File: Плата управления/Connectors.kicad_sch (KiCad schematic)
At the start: 9 parts, among them J1 A, J2 B, J3 C, J4 CAN2, J5 Conn_02x07_Odd_Even, J6 CAN1, J7 RS-485, J8 Conn_02x10_Odd_Even, J9 Inputs

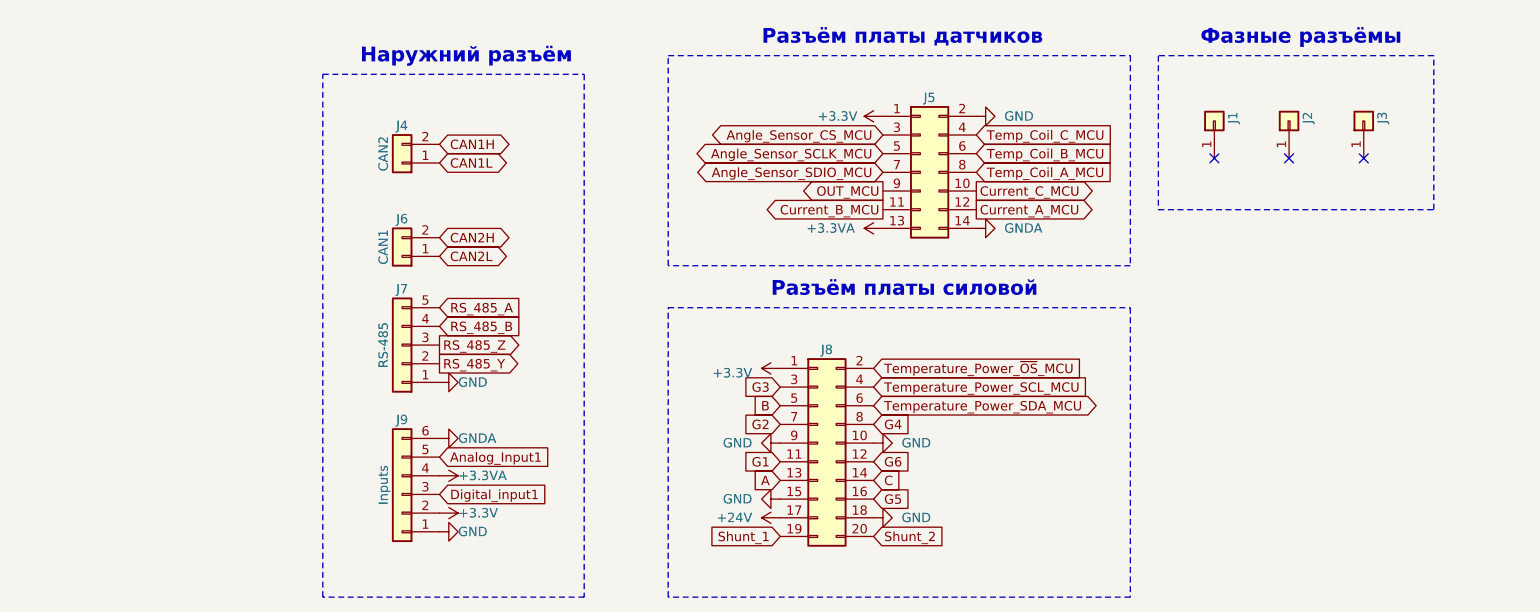
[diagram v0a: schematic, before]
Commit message: Версия под отчёт
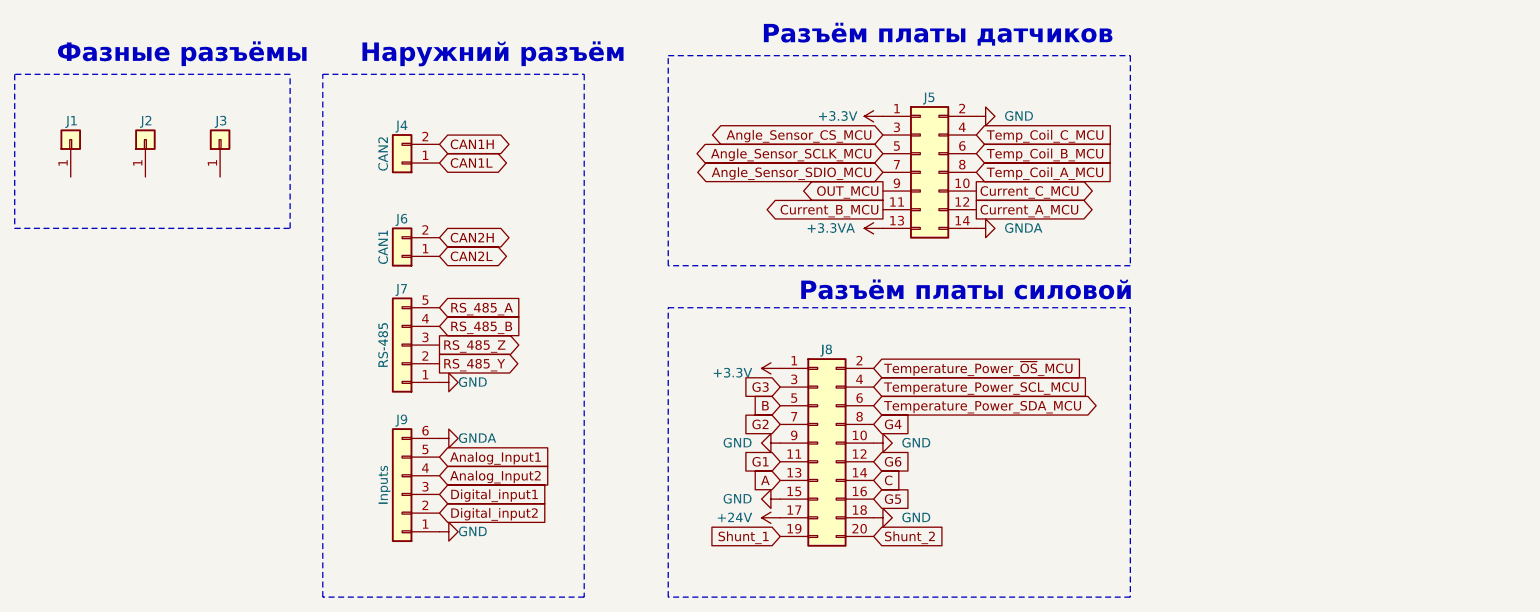
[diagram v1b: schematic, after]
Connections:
- net +3.3V: no longer J9.2 (Pin_2)
- net +3.3VA: no longer J9.4 (Pin_4)
- new net Analog_Input2: J9.4 (Pin_4)
- new net Digital_input2: J9.2 (Pin_2)
- no-connect marks 3 -> 0
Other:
- moved on the sheet: J1, J2, J3
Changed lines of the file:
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@@
     (comment 1 "МПСТ.76721.758764.02.Э3.М")
   )
-  (no_connect (at 210.82 86.995))
-  (no_connect (at 220.98 86.995))
-  (no_connect (at 200.66 86.995))
   (rectangle (start 126.365 107.315) (end 189.23 146.685)
     (stroke (width 0) (type dash))
     (fill (type none))
   )
-  (rectangle (start 230.505 73.025) (end 193.04 93.98)
+  (rectangle (start 74.93 75.565) (end 37.465 96.52)
     (stroke (width 0) (type dash))
     (fill (type none))
@@
     (fill (type none))
   )
-  (text "Фазные разъёмы" (at 198.755 71.755 0)
-    (effects (font (size 2 2) (thickness 0.4) bold) (justify left bottom))
+  (text "Фазные разъёмы" (at 43.18 74.295 0)
+    (effects (font (size 2.5 2.5) (thickness 0.4) bold) (justify left bottom))
   )
   (text "Разъём платы датчиков\n" (at 139.065 71.755 0)
-    (effects (font (size 2 2) (thickness 0.4) bold) (justify left bottom))
+    (effects (font (size 2.5 2.5) (thickness 0.4) bold) (justify left bottom))
   )
   (text "Наружний разъём\n" (at 84.455 74.295 0)
-    (effects (font (size 2 2) (thickness 0.4) bold) (justify left bottom))
-  )
-  (text "Разъём платы силовой\n" (at 140.335 106.045 0)
-    (effects (font (size 2 2) (thickness 0.4) bold) (justify left bottom))
+    (effects (font (size 2.5 2.5) (thickness 0.4) bold) (justify left bottom))
+  )
+  (text "Разъём платы силовой\n" (at 144.145 106.68 0)
+    (effects (font (size 2.5 2.5) (thickness 0.4) bold) (justify left bottom))
   )
   (global_label "G3" (shape input) (at 141.605 118.11 180) (fields_autoplaced)
@@
     )
   )
+  (global_label "Digital_input1" (shape input) (at 95.25 132.715 0) (fields_autoplaced)
+    (effects (font (size 1.27 1.27)) (justify left))
+    (property "Intersheetrefs" "${INTERSHEET_REFS}" (at 111.3583 132.715 0)
+      (effects (font (size 1.27 1.27)) (justify left) hide)
+    )
+  )
   (global_label "Temp_Coil_A_MCU" (shape input) (at 168.275 88.9 0) (fields_autoplaced)
     (effects (font (size 1.27 1.27)) (justify left))
@@
     )
   )
+  (global_label "Analog_Input2" (shape input) (at 95.25 130.175 0) (fields_autoplaced)
+    (effects (font (size 1.27 1.27)) (justify left))
+    (property "Intersheetrefs" "${INTERSHEET_REFS}" (at 109.0703 130.175 0)
+      (effects (font (size 1.27 1.27)) (justify left) hide)
+    )
+  )
   (global_label "OUT_MCU" (shape output) (at 155.575 91.44 180) (fields_autoplaced)
     (effects (font (size 1.27 1.27)) (justify right))
@@
     )
   )
-  (global_label "Digital_input1" (shape input) (at 95.25 132.715 0) (fields_autoplaced)
-    (effects (font (size 1.27 1.27)) (justify left))
-    (property "Intersheetrefs" "${INTERSHEET_REFS}" (at 111.3583 132.715 0)
+  (global_label "Digital_input2" (shape input) (at 95.25 135.255 0) (fields_autoplaced)
+    (effects (font (size 1.27 1.27)) (justify left))
+    (property "Intersheetrefs" "${INTERSHEET_REFS}" (at 108.6894 135.255 0)
       (effects (font (size 1.27 1.27)) (justify left) hide)
     )
@@
         (path "/75f4c67c-bbde-4446-8f82-67797a1b269f/f5e732cc-be4b-4207-bf28-0691ff32221d"
           (reference "#PWR031") (unit 1)
-        )
-      )
-      (project "Силовая плата"
-        (path "/96c6fc92-8ec6-44f7-b0dc-9ad8f1acea09/a27b443f-c036-4fd6-934c-6ea912709de0"
-          (reference "#PWR042") (unit 1)
-        )
-      )
-    )
-  )
-  (symbol (lib_id "power:+3.3V") (at 95.25 135.255 270) (unit 1)
-    (in_bom yes) (on_board yes) (dnp no)
-    (property "Reference" "#PWR038" (at 91.44 135.255 0)
-      (effects (font (size 1.27 1.27)) hide)
-    )
-    (property "Value" "+3.3V" (at 97.79 135.255 90)
-      (effects (font (size 1.27 1.27)) (justify left))
-    )
-    (property "Footprint" "" (at 95.25 135.255 0)
-      (effects (font (size 1.27 1.27)) hide)
-    )
-    (property "Datasheet" "" (at 95.25 135.255 0)
-      (effects (font (size 1.27 1.27)) hide)
-    )
-    (pin "1")
-    (instances
-      (project "Плата управления"
-        (path "/75f4c67c-bbde-4446-8f82-67797a1b269f/f5e732cc-be4b-4207-bf28-0691ff32221d"
-          (reference "#PWR038") (unit 1)
         )
       )
@@
     )
   )
-  (symbol (lib_id "Connector_Generic:Conn_01x01") (at 210.82 81.915 90) (unit 1)
+  (symbol (lib_id "Connector_Generic:Conn_01x01") (at 55.245 84.455 90) (unit 1)
     (in_bom yes) (on_board yes) (dnp no)
-    (property "Reference" "J2" (at 213.36 80.645 0)
+    (property "Reference" "J2" (at 54.61 81.915 90)
       (effects (font (size 1.27 1.27)) (justify right))
     )
-    (property "Value" "B" (at 213.36 83.185 90)
-      (effects (font (size 1.27 1.27)) (justify right) hide)
-    )
-    (property "Footprint" "Connector_My:Power_Wire" (at 210.82 81.915 0)
-      (effects (font (size 1.27 1.27)) hide)
-    )
-    (property "Datasheet" "~" (at 210.82 81.915 0)
+    (property "Value" "B" (at 57.785 85.725 90)
+      (effects (font (size 1.27 1.27)) (justify right) hide)
+    )
+    (property "Footprint" "Connector_My:Power_Wire" (at 55.245 84.455 0)
+      (effects (font (size 1.27 1.27)) hide)
+    )
+    (property "Datasheet" "~" (at 55.245 84.455 0)
       (effects (font (size 1.27 1.27)) hide)
     )
@@
     )
   )
-  (symbol (lib_id "Connector_Generic:Conn_01x01") (at 220.98 81.915 90) (unit 1)
+  (symbol (lib_id "Connector_Generic:Conn_01x01") (at 65.405 84.455 90) (unit 1)
     (in_bom yes) (on_board yes) (dnp no)
-    (property "Reference" "J3" (at 223.52 80.645 0)
+    (property "Reference" "J3" (at 64.77 81.915 90)
       (effects (font (size 1.27 1.27)) (justify right))
     )
-    (property "Value" "C" (at 223.52 83.185 90)
-      (effects (font (size 1.27 1.27)) (justify right) hide)
-    )
-    (property "Footprint" "Connector_My:Power_Wire" (at 220.98 81.915 0)
-      (effects (font (size 1.27 1.27)) hide)
-    )
-    (property "Datasheet" "~" (at 220.98 81.915 0)
+    (property "Value" "C" (at 67.945 85.725 90)
+      (effects (font (size 1.27 1.27)) (justify right) hide)
+    )
+    (property "Footprint" "Connector_My:Power_Wire" (at 65.405 84.455 0)
+      (effects (font (size 1.27 1.27)) hide)
+    )
+    (property "Datasheet" "~" (at 65.405 84.455 0)
       (effects (font (size 1.27 1.27)) hide)
     )
@@
     )
   )
-  (symbol (lib_id "Connector_Generic:Conn_01x01") (at 200.66 81.915 90) (unit 1)
+  (symbol (lib_id "Connector_Generic:Conn_01x01") (at 45.085 84.455 90) (unit 1)
     (in_bom yes) (on_board yes) (dnp no)
-    (property "Reference" "J1" (at 203.2 80.645 0)
+    (property "Reference" "J1" (at 44.45 81.915 90)
       (effects (font (size 1.27 1.27)) (justify right))
     )
-    (property "Value" "A" (at 203.2 83.185 90)
-      (effects (font (size 1.27 1.27)) (justify right) hide)
-    )
-    (property "Footprint" "Connector_My:Power_Wire" (at 200.66 81.915 0)
-      (effects (font (size 1.27 1.27)) hide)
-    )
-    (property "Datasheet" "~" (at 200.66 81.915 0)
+    (property "Value" "A" (at 47.625 85.725 90)
+      (effects (font (size 1.27 1.27)) (justify right) hide)
+    )
+    (property "Footprint" "Connector_My:Power_Wire" (at 45.085 84.455 0)
+      (effects (font (size 1.27 1.27)) hide)
+    )
+    (property "Datasheet" "~" (at 45.085 84.455 0)
       (effects (font (size 1.27 1.27)) hide)
     )
@@
         )
       )
-    )
-  )
-  (symbol (lib_id "power:+3.3VA") (at 95.25 130.175 270) (unit 1)
-    (in_bom yes) (on_board yes) (dnp no)
-    (property "Reference" "#PWR036" (at 91.44 130.175 0)
-      (effects (font (size 1.27 1.27)) hide)
-    )
-    (property "Value" "+3.3VA" (at 97.79 130.175 90)
-      (effects (font (size 1.27 1.27)) (justify left))
-    )
-    (property "Footprint" "" (at 95.25 130.175 0)
-      (effects (font (size 1.27 1.27)) hide)
-    )
-    (property "Datasheet" "" (at 95.25 130.175 0)
-      (effects (font (size 1.27 1.27)) hide)
-    )
-    (pin "1")
-    (instances
-      (project "Плата управления"
-        (path "/75f4c67c-bbde-4446-8f82-67797a1b269f/f5e732cc-be4b-4207-bf28-0691ff32221d"
-          (reference "#PWR036") (unit 1)
-        )
-      )
